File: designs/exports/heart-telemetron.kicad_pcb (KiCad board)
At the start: 2 copper layers, 45 x 40 mm, 4 parts

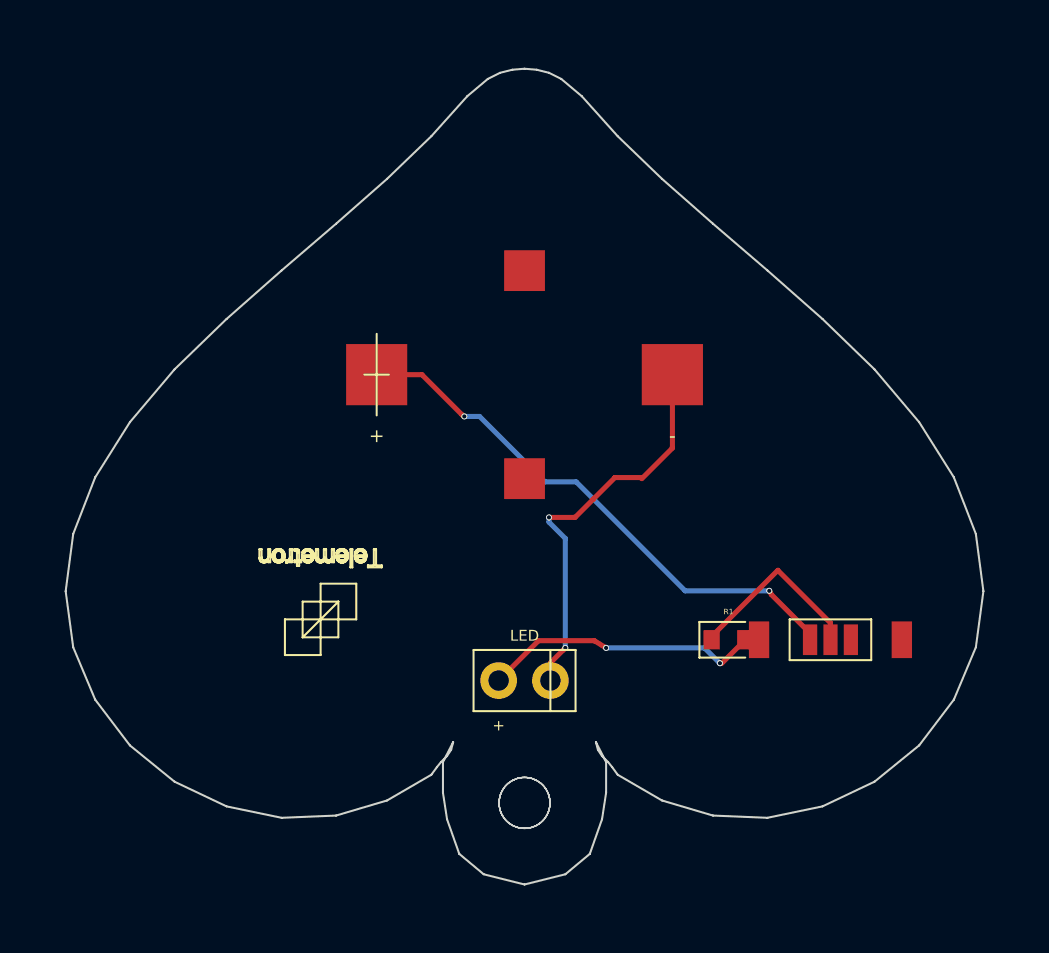
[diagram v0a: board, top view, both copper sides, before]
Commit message: Re-export all 4 variants: SVGs, gerbers, KiCad files
All designs current with CAD heart outline, updated components, and logos.

Co-Authored-By: Claude Opus 4.6 (1M context) <noreply@anthropic.com>
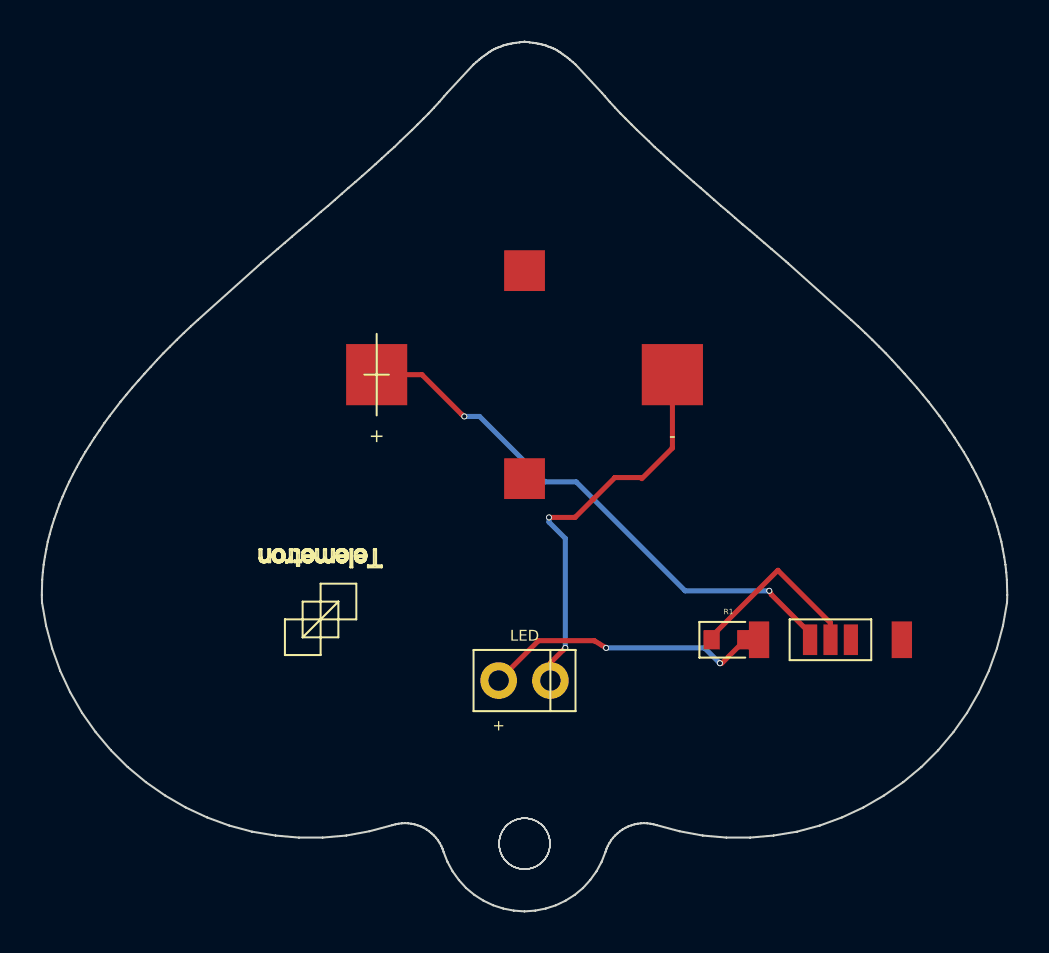
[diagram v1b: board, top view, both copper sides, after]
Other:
- board size 45 x 40 mm -> 47.3 x 42.6 mm
